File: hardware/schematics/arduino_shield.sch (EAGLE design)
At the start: 41 parts, among them IC1 LM358KIT, IC2 MAX548, Q1 IRL520N-H, Q2 IRL520N-H, Q3 IRF9Z24, Q4 IRL520N-H, Q5 IRL520N-H, Q6 IRF9Z24, X5 Channel A, X6 Channel B

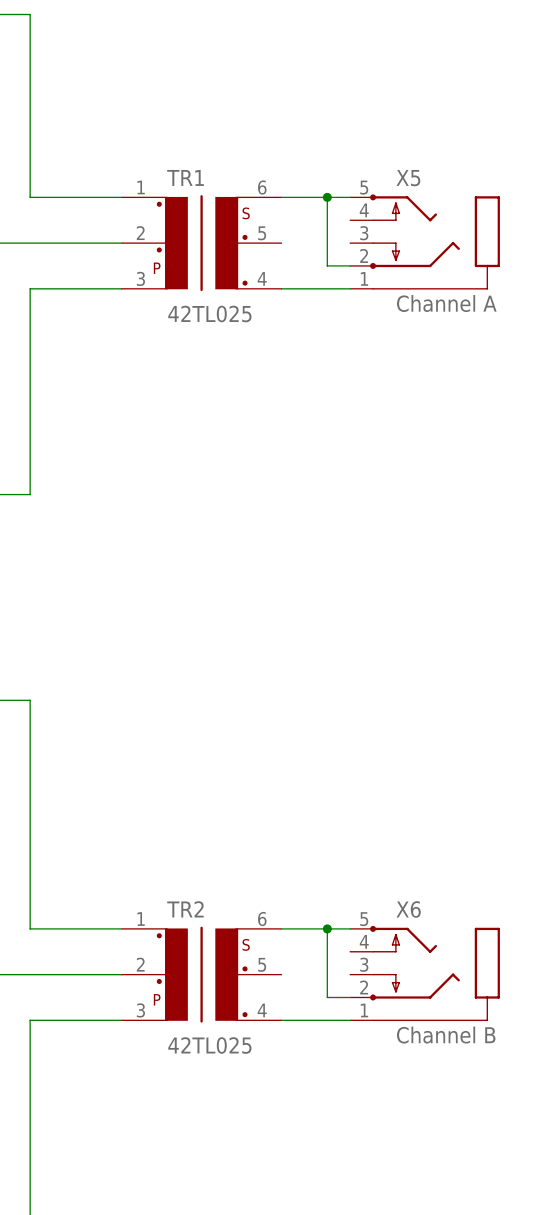
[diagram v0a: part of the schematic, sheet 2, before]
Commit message: update
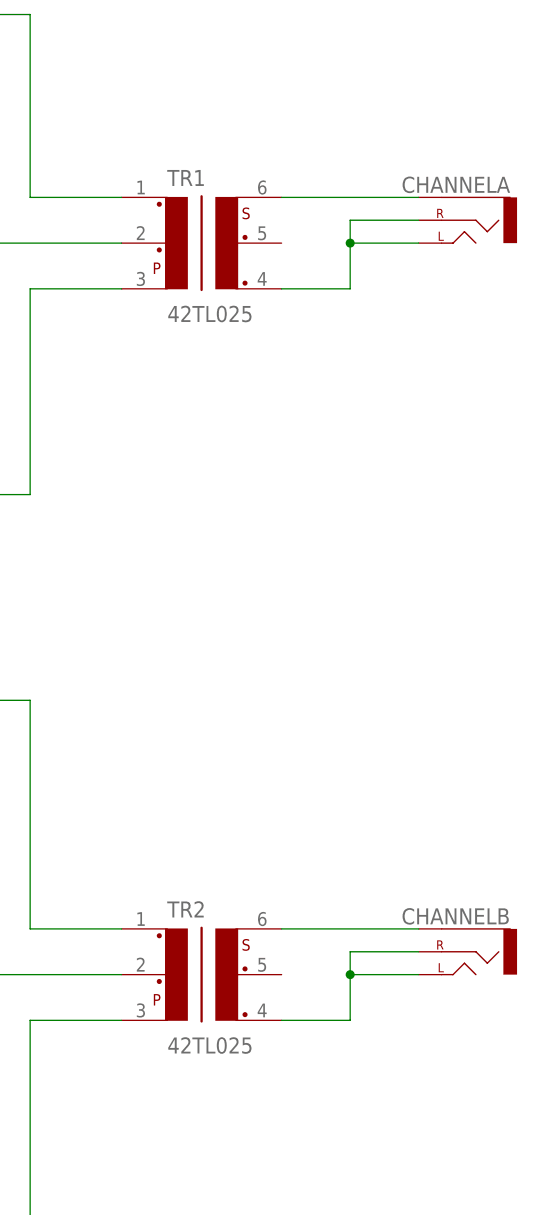
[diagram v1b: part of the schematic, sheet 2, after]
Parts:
- removed X5: Channel A, adafruit:STEREOJACK
- removed X6: Channel B, adafruit:STEREOJACK
- added CHANNELA, CHANNELB: (no value), SparkFun-Connectors:AUDIO-JACK2.5MM
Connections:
- net N$1: now also CHANNELA.SLEEVE, TR1.6; no longer TR1.4, X5.1
- net N$2: now also CHANNELB.SLEEVE, TR2.6; no longer TR1.6, X5.2, X5.5
- net N$3: now also CHANNELB.LEFT, CHANNELB.RIGHT, TR2.4; no longer TR2.6, X6.2, X6.5
- net N$4: now also CHANNELA.LEFT, CHANNELA.RIGHT, TR1.4; no longer TR2.4, X6.1
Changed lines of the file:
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@@
 <?xml version="1.0" encoding="utf-8"?>
 <!DOCTYPE eagle SYSTEM "eagle.dtd">
-<eagle version="7.1.0">
+<eagle version="7.3.0">
 <drawing>
 <settings>
@@
 <part name="GND15" library="supply1" deviceset="GND" device=""/>
 <part name="R22" library="eagle-ltspice" deviceset="R" device="" value="100k"/>
-<part name="X5" library="adafruit" deviceset="STEREOJACK" device="" value="Channel A"/>
-<part name="X6" library="adafruit" deviceset="STEREOJACK" device="" value="Channel B"/>
 <part name="GND21" library="supply1" deviceset="GND" device=""/>
 <part name="U$3" library="adafruit" deviceset="ARDUINO" device="UNO"/>
@@
 <part name="JP2" library="SparkFun-Connectors" deviceset="M02" device="3.5MM"/>
 <part name="GND4" library="supply1" deviceset="GND" device=""/>
+<part name="CHANNELA" library="SparkFun-Connectors" deviceset="AUDIO-JACK" device="2.5MM"/>
+<part name="CHANNELB" library="SparkFun-Connectors" deviceset="AUDIO-JACK" device="2.5MM"/>
 </parts>
 <sheets>
@@
 <instance part="R22" gate="G$1" x="66.04" y="55.88"/>
 <instance part="FRAME6" gate="G$1" x="0" y="0"/>
-<instance part="X5" gate="1" x="215.9" y="149.86"/>
-<instance part="X6" gate="1" x="215.9" y="68.58"/>
 <instance part="GND21" gate="1" x="134.62" y="10.16"/>
 <instance part="P+7" gate="1" x="88.9" y="86.36"/>
@@
 <instance part="P+10" gate="1" x="50.8" y="111.76"/>
 <instance part="GND3" gate="1" x="15.24" y="86.36"/>
+<instance part="CHANNELA" gate="G$1" x="215.9" y="149.86" rot="MR0"/>
+<instance part="CHANNELB" gate="G$1" x="215.9" y="68.58" rot="MR0"/>
 </instances>
 <busses>
@@
 <wire x1="132.08" y1="48.26" x2="132.08" y2="45.72" width="0.1524" layer="91"/>
 <junction x="132.08" y="45.72"/>
-</segment>
-</net>
-<net name="N$1" class="0">
-<segment>
-<pinref part="TR1" gate="G$1" pin="4"/>
-<pinref part="X5" gate="1" pin="1"/>
-<wire x1="195.58" y1="142.24" x2="203.2" y2="142.24" width="0.1524" layer="91"/>
-</segment>
-</net>
-<net name="N$2" class="0">
-<segment>
-<pinref part="TR1" gate="G$1" pin="6"/>
-<pinref part="X5" gate="1" pin="5"/>
-<wire x1="195.58" y1="152.4" x2="200.66" y2="152.4" width="0.1524" layer="91"/>
-<wire x1="203.2" y1="152.4" x2="200.66" y2="152.4" width="0.1524" layer="91"/>
-<wire x1="200.66" y1="152.4" x2="200.66" y2="144.78" width="0.1524" layer="91"/>
-<pinref part="X5" gate="1" pin="2"/>
-<wire x1="200.66" y1="144.78" x2="203.2" y2="144.78" width="0.1524" layer="91"/>
-<junction x="200.66" y="152.4"/>
-</segment>
-</net>
-<net name="N$3" class="0">
-<segment>
-<pinref part="TR2" gate="G$1" pin="6"/>
-<pinref part="X6" gate="1" pin="5"/>
-<wire x1="195.58" y1="71.12" x2="200.66" y2="71.12" width="0.1524" layer="91"/>
-<wire x1="203.2" y1="71.12" x2="200.66" y2="71.12" width="0.1524" layer="91"/>
-<wire x1="200.66" y1="71.12" x2="200.66" y2="63.5" width="0.1524" layer="91"/>
-<pinref part="X6" gate="1" pin="2"/>
-<wire x1="200.66" y1="63.5" x2="203.2" y2="63.5" width="0.1524" layer="91"/>
-<junction x="200.66" y="71.12"/>
-</segment>
-</net>
-<net name="N$4" class="0">
-<segment>
-<pinref part="X6" gate="1" pin="1"/>
-<pinref part="TR2" gate="G$1" pin="4"/>
-<wire x1="203.2" y1="60.96" x2="195.58" y2="60.96" width="0.1524" layer="91"/>
 </segment>
 </net>
@@
 </segment>
 </net>
+<net name="N$1" class="0">
+<segment>
+<pinref part="CHANNELA" gate="G$1" pin="SLEEVE"/>
+<pinref part="TR1" gate="G$1" pin="6"/>
+<wire x1="210.82" y1="152.4" x2="195.58" y2="152.4" width="0.1524" layer="91"/>
+</segment>
+</net>
+<net name="N$2" class="0">
+<segment>
+<pinref part="CHANNELB" gate="G$1" pin="SLEEVE"/>
+<pinref part="TR2" gate="G$1" pin="6"/>
+<wire x1="210.82" y1="71.12" x2="195.58" y2="71.12" width="0.1524" layer="91"/>
+</segment>
+</net>
+<net name="N$3" class="0">
+<segment>
+<pinref part="CHANNELB" gate="G$1" pin="RIGHT"/>
+<wire x1="210.82" y1="68.58" x2="203.2" y2="68.58" width="0.1524" layer="91"/>
+<wire x1="203.2" y1="68.58" x2="203.2" y2="66.04" width="0.1524" layer="91"/>
+<pinref part="TR2" gate="G$1" pin="4"/>
+<wire x1="203.2" y1="66.04" x2="203.2" y2="60.96" width="0.1524" layer="91"/>
+<wire x1="203.2" y1="60.96" x2="195.58" y2="60.96" width="0.1524" layer="91"/>
+<pinref part="CHANNELB" gate="G$1" pin="LEFT"/>
+<wire x1="210.82" y1="66.04" x2="203.2" y2="66.04" width="0.1524" layer="91"/>
+<junction x="203.2" y="66.04"/>
+</segment>
+</net>
+<net name="N$4" class="0">
+<segment>
+<pinref part="CHANNELA" gate="G$1" pin="RIGHT"/>
+<wire x1="210.82" y1="149.86" x2="203.2" y2="149.86" width="0.1524" layer="91"/>
+<wire x1="203.2" y1="149.86" x2="203.2" y2="147.32" width="0.1524" layer="91"/>
+<pinref part="TR1" gate="G$1" pin="4"/>
+<wire x1="203.2" y1="147.32" x2="203.2" y2="142.24" width="0.1524" layer="91"/>
+<wire x1="203.2" y1="142.24" x2="195.58" y2="142.24" width="0.1524" layer="91"/>
+<pinref part="CHANNELA" gate="G$1" pin="LEFT"/>
+<wire x1="210.82" y1="147.32" x2="203.2" y2="147.32" width="0.1524" layer="91"/>
+<junction x="203.2" y="147.32"/>
+</segment>
+</net>
